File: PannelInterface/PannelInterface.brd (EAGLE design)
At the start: 45 x 100 mm, 10 parts, among them IC2 LM2575D2T-012

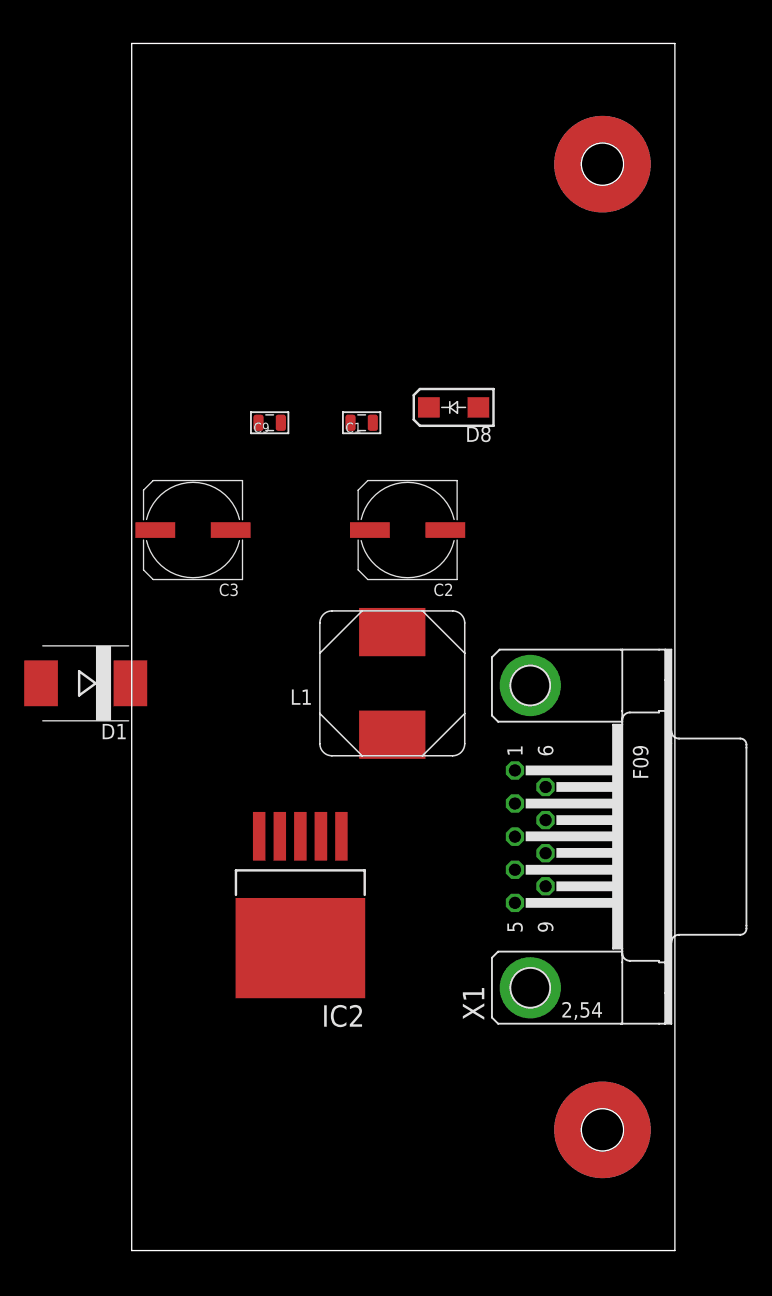
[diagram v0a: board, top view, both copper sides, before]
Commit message: PI change
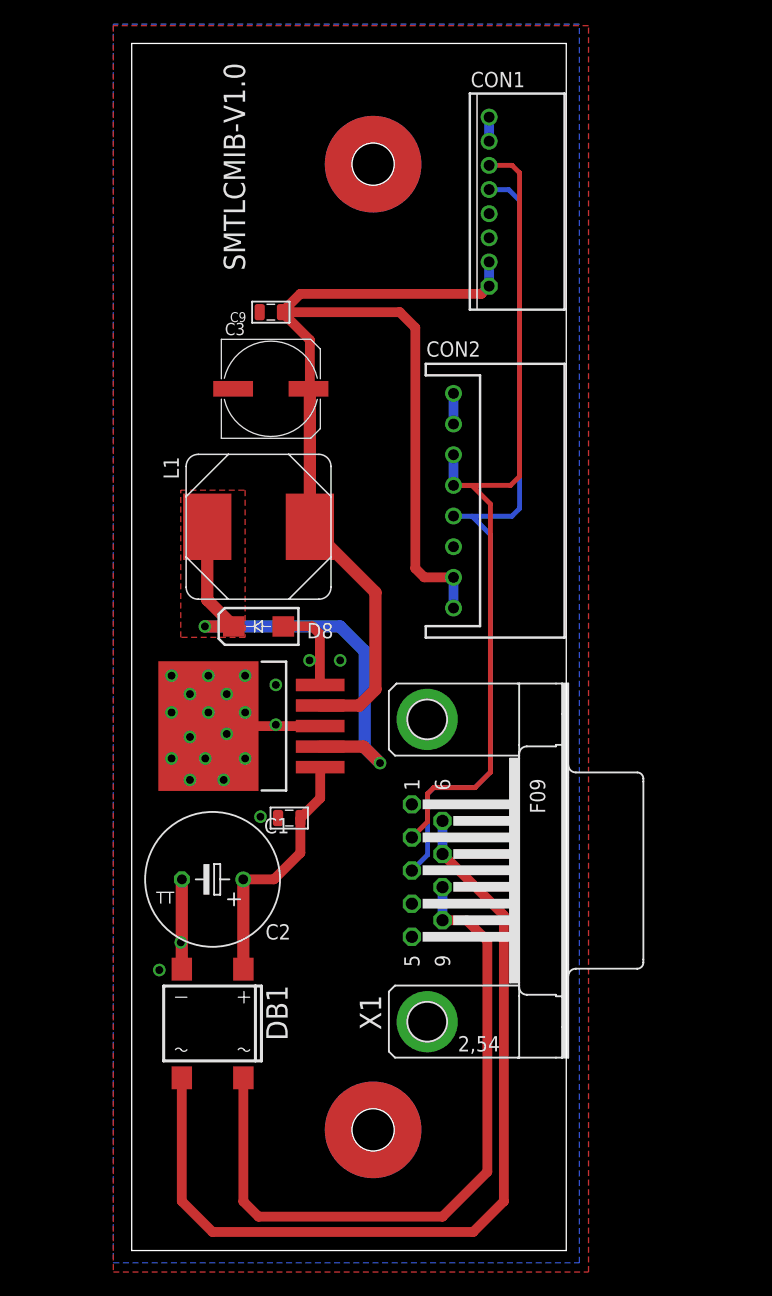
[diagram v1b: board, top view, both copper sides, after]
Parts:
- removed D1: SMDJ30A, SHMT:SMC
- added CON1: PH-8AW, prj-pannel_interface:PH-8AW
- added CON2: XH-8AW, prj-pannel_interface:XH-8AW
- added DB1: DB207S, prj-pannel_interface:DBS
- added LOGO1: SY-LOGO_BOTTOM, LOGO:SY-LOGO_BOTTOM
- C2: device rcl:UD-8X10_NICHICON -> rcl:TT5D11
- L1: value 330uH/2A_RH125 -> 330uH/2A_RH127
- moved C1 33.3 mm to (13.1, 35.8)
- moved C2 33.1 mm to (6.70, 30.8)
- moved D8 24.3 mm to (10.5, 51.7)
- moved L1 17.1 mm to (10.5, 60.0), turned to 90 degrees
- moved IC2 14.7 mm to (10.5, 43.5), turned to 90 degrees
- moved C3 13.4 mm to (11.5, 71.4), turned to 0 degrees
- moved C9 9.16 mm to (11.5, 77.7)
- moved X1 8.99 mm to (24.5, 31.5)
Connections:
- new net AC1: DB1.AC2, X1.6, X1.7
- new net AC2: DB1.AC1, X1.8, X1.9
- new net RXD: CON1.6, CON2.5, CON2.6, X1.2
- new net TXD: CON1.5, CON2.4, X1.3
- net +12V: now also CON1.1, CON1.2, CON2.1, CON2.2
- net GND: now also CON1.7, CON1.8, CON2.7, CON2.8, DB1.-, X1.G1, X1.G2; no longer D1.A
- net N$1: now also DB1.+; no longer D1.C
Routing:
- net +12V: track 0.00 -> 97.3 mm
- net AC1: track 0.00 -> 72.6 mm
- net RXD: track 0.00 -> 72.3 mm
- net TXD: track 0.00 -> 68.9 mm
- net AC2: track 0.00 -> 58.8 mm
- net N$34: track 0.00 -> 41.0 mm, vias 0 -> 2
- net GND: track 0.00 -> 28.8 mm, vias 0 -> 22
- net N$1: track 0.00 -> 20.9 mm
- added copper zone on layer 1, net GND
- added copper zone on layer 16, net GND
- added copper zone on layer 1, net N$34
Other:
- board size 45 x 100 mm -> 36 x 100 mm
- board text added: "SMTLCMIB-V1.0"
